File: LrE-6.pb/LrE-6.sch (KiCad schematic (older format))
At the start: 115 parts, among them J1 USB_B_Micro, J2 SM06B-SRSS-TB, J3 LP_Header_02x03, J4 LP_Header_01x02, Q1 2N7002, Q11 2N7002, SW1 SW_Push_45deg, SW10 SW_Push_45deg, SW11 Rotary_Encoder_Switch, SW12 Rotary_Encoder_Switch, SW13 Rotary_Encoder_Switch, SW14 Rotary_Encoder_Switch, SW15 Rotary_Encoder_Switch, SW16 Rotary_Encoder_Switch, SW2 SW_Push_45deg, SW3 SW_Push_45deg, SW4 SW_Push_45deg, SW5 SW_Push_45deg, SW6 SW_Push_45deg, SW7 SW_Push_45deg, SW8 SW_Push_45deg, SW9 SW_Push_45deg, U1 STM32F072C8Tx, U2 ESP-WROOM-02, U3 AQM0802-FLW-GBW, U4 SPX3819M5-L3-3TR

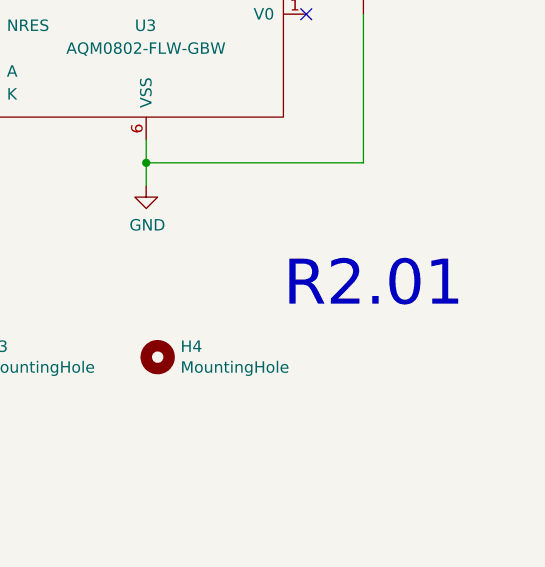
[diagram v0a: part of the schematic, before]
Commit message: 0.22-pre1
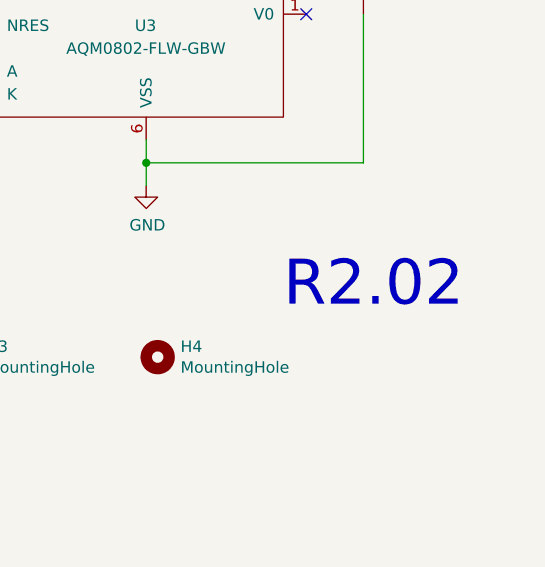
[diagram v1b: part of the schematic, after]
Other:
- note added: "R2.02"
- note removed: "R2.01"
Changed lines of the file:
@@
 	12250 4150 12700 4150
 Text Notes 15150 9550 0    197  ~ 0
-R2.01
+R2.02
 Wire Wire Line
 	11750 3250 12700 3250
